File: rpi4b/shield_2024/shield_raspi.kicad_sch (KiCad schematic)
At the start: 12 parts, among them J1 VL53, J10 LED, J11 LED, J2 LED, J3 LED, J4 Conn_02x20_Odd_Even, J5 Conn_01x04_Pin, J6 Conn_01x04_Pin, J7 VL53, J8 VL53, J9 VL53, U1 RASPBERRY_PI_4B_4GB

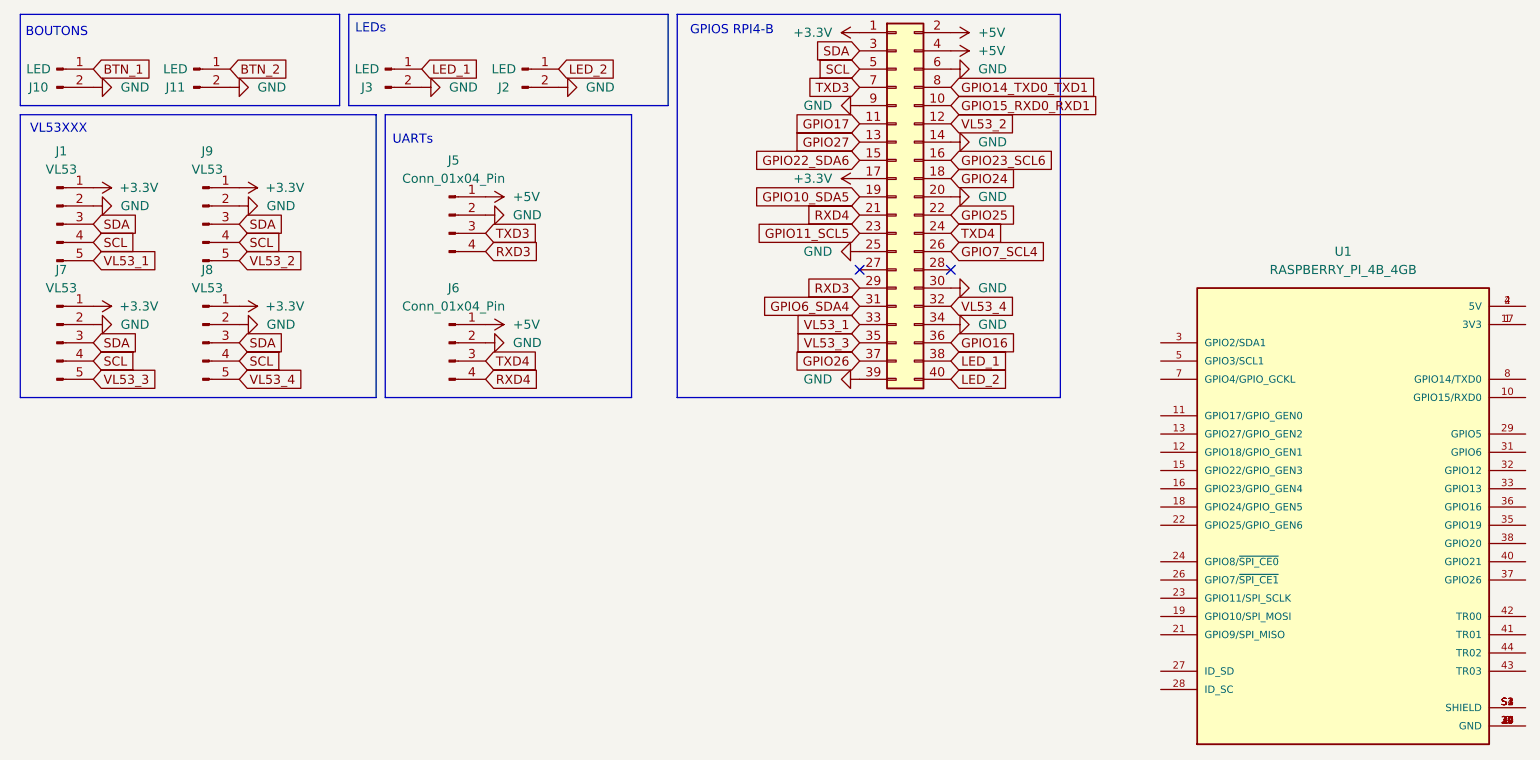
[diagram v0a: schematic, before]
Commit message: placement composant
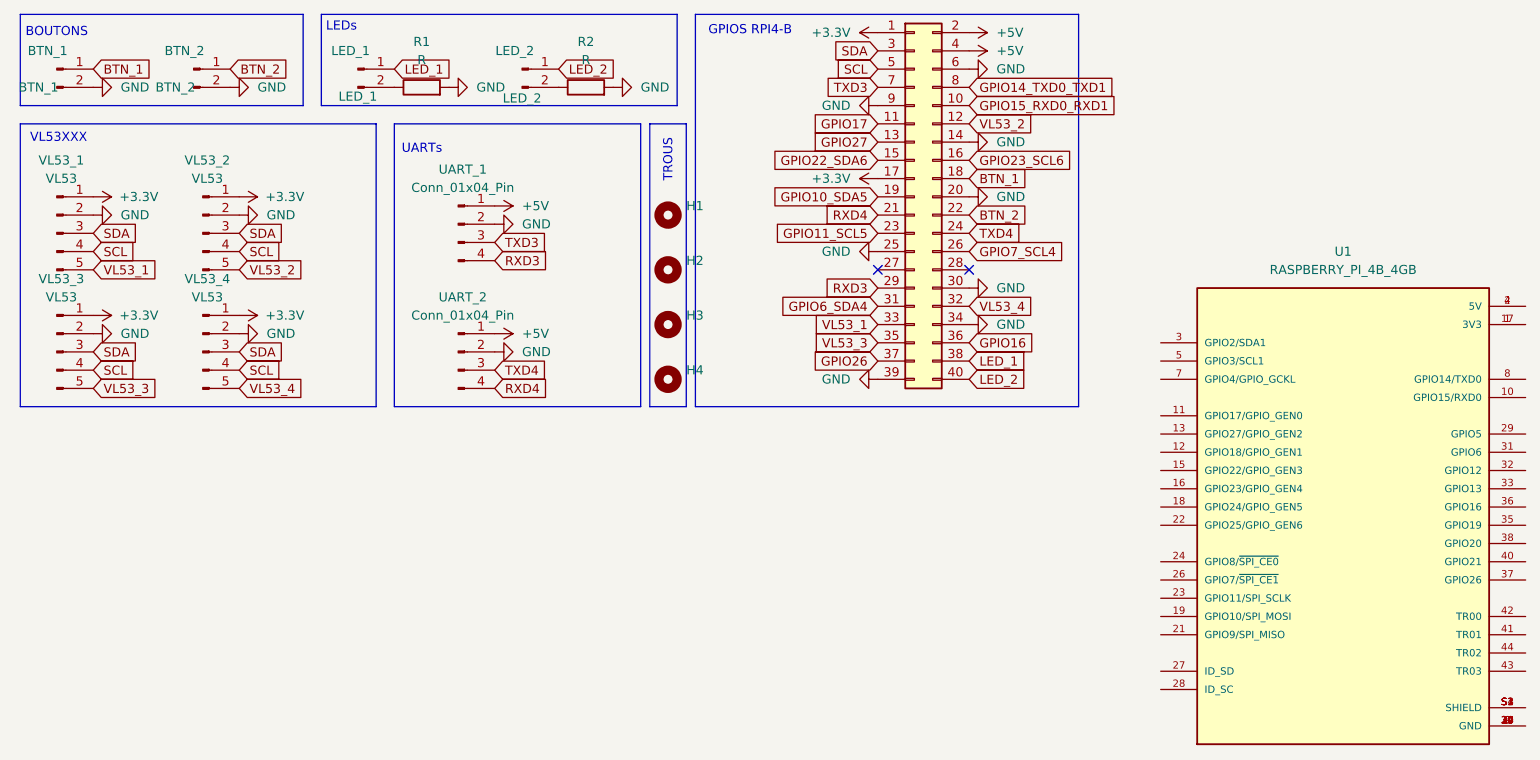
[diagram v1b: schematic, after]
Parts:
- added H1, H2, H3, H4: MountingHole, MountingHole:MountingHole_3.2mm_M3, symbol Mechanical:MountingHole
- added R1, R2: R, Resistor_SMD:R_0603_1608Metric, symbol Device:R
- BTN_1: renamed from J10; value LED -> BTN_1
- BTN_2: renamed from J11; value LED -> BTN_2
- LED_1: renamed from J3; value LED -> LED_1
- LED_2: renamed from J2; value LED -> LED_2
- renumbered J5 to UART_1, J6 to UART_2, J1 to VL53_1, J9 to VL53_2, J7 to VL53_3, J8 to VL53_4
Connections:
- net GPIO24 is gone; now on net BTN_1: J4.18 (Pin_18)
- net GPIO25 is gone; now on net BTN_2: J4.22 (Pin_22)
- net GND: now also R1.2, R2.2; no longer LED_1.2 (Pin_2), LED_2.2 (Pin_2)
- new net: LED_1.2 (Pin_2), R1.1
- new net: LED_2.2 (Pin_2), R2.1
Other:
- note added: "TROUS"
- moved on the sheet: LED_1, UART_1, UART_2, VL53_1, VL53_2, VL53_3, VL53_4
